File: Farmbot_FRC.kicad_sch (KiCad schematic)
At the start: 3 parts, among them J1 XT60-M, U1 NEO-6M-GPS

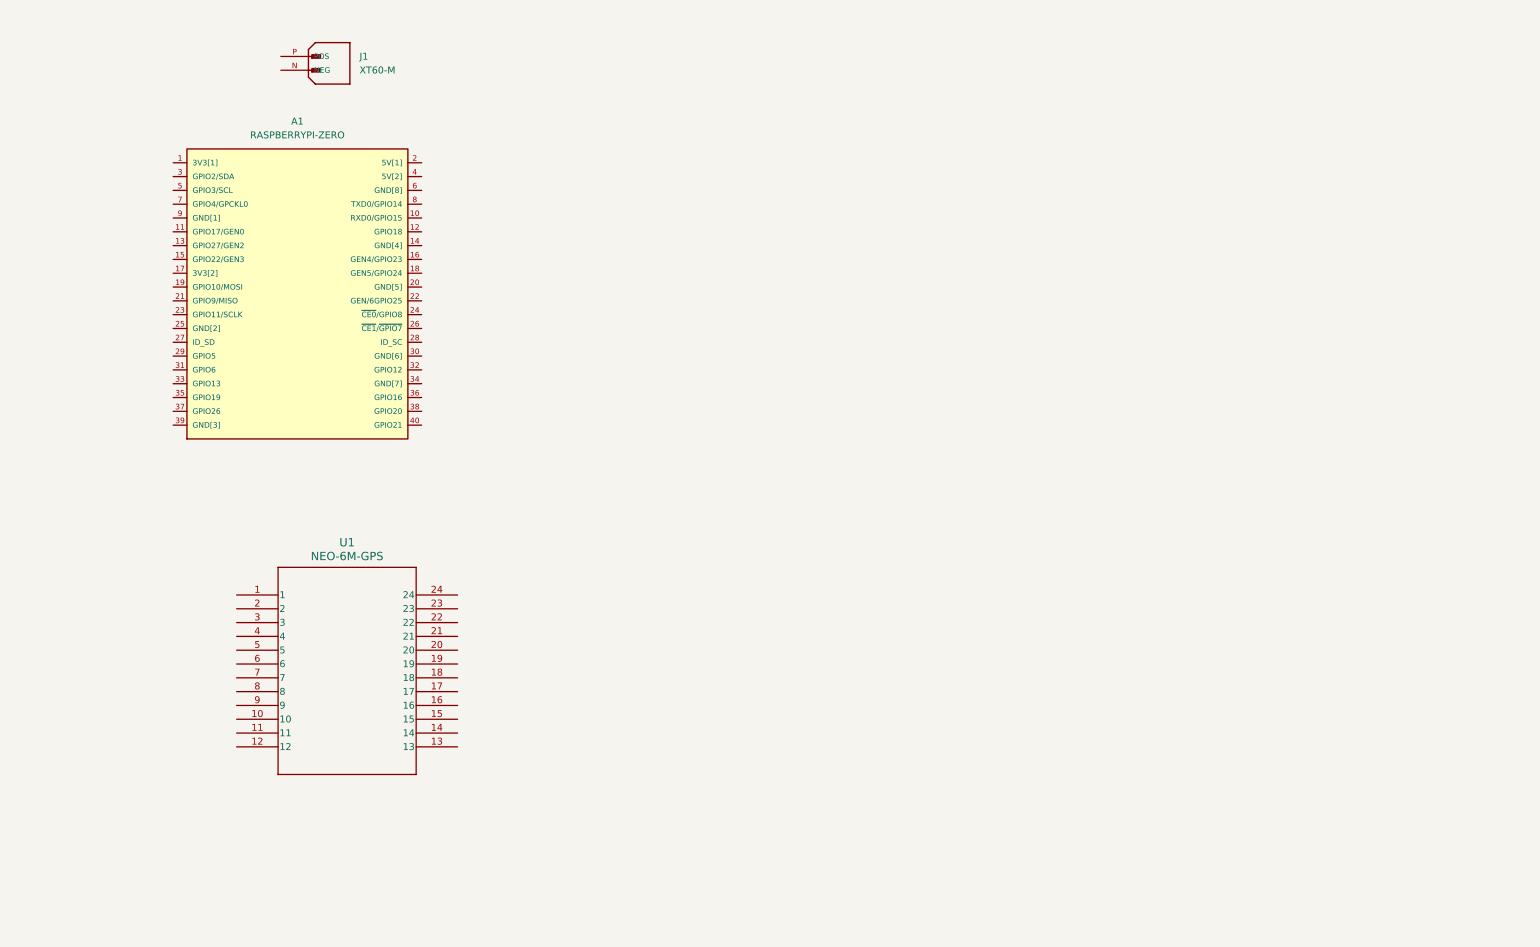
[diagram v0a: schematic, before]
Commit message: Added basic components
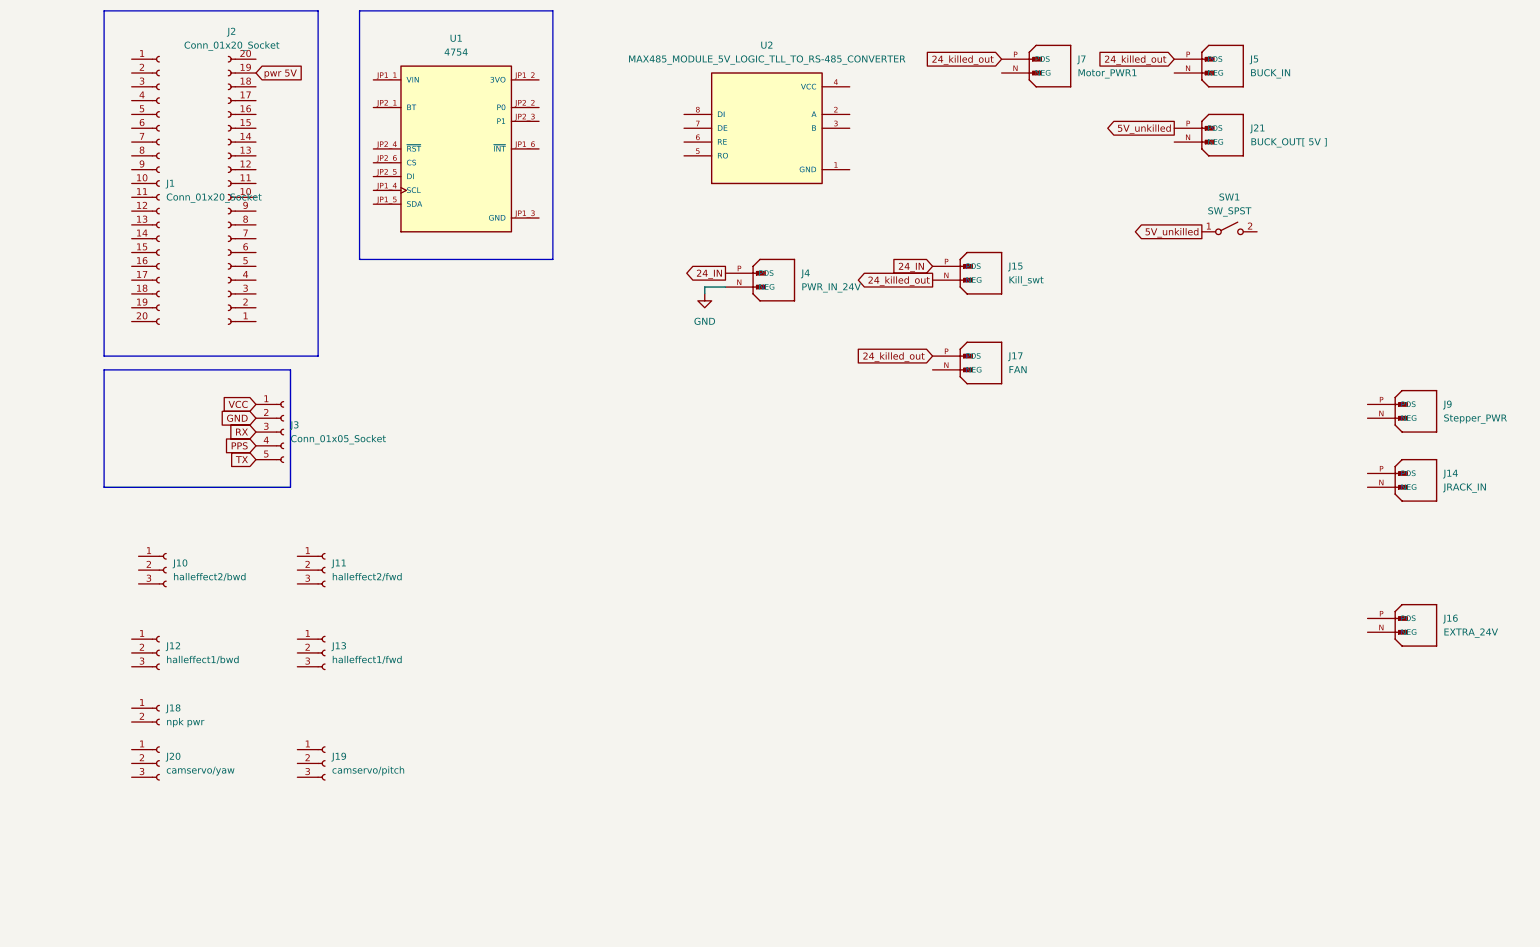
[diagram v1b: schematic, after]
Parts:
- removed A1: RASPBERRYPI-ZERO, RASPBERRYPI-ZERO:RASPBERRYPI-ZERO_RPI-ZERO, symbol RASPBERRYPI-ZERO:RASPBERRYPI-ZERO
- removed J1: XT60-M, XT60-M:AMASS_XT60-M, symbol XT60-M:XT60-M
- removed U1: NEO-6M-GPS, SON_6M-GPS_UBL, symbol gps neo 6m:NEO-6M-GPS
- added J1, J2: Conn_01x20_Socket, symbol Connector:Conn_01x20_Socket
- added J10: halleffect2/bwd, symbol Connector:Conn_01x03_Socket
- added J11: halleffect2/fwd, symbol Connector:Conn_01x03_Socket
- added J12: halleffect1/bwd, symbol Connector:Conn_01x03_Socket
- added J13: halleffect1/fwd, symbol Connector:Conn_01x03_Socket
- added J14: JRACK_IN, XT60-M:AMASS_XT60-M, symbol XT60-M:XT60-M
- added J15: Kill_swt, XT60-M:AMASS_XT60-M, symbol XT60-M:XT60-M
- added J16: EXTRA_24V, XT60-M:AMASS_XT60-M, symbol XT60-M:XT60-M
- added J17: FAN, XT60-M:AMASS_XT60-M, symbol XT60-M:XT60-M
- added J18: npk pwr, symbol Connector:Conn_01x02_Socket
- added J19: camservo/pitch, symbol Connector:Conn_01x03_Socket
- added J20: camservo/yaw, symbol Connector:Conn_01x03_Socket
- added J21: BUCK_OUT[ 5V ], XT60-M:AMASS_XT60-M, symbol XT60-M:XT60-M
- added J3: Conn_01x05_Socket, symbol Connector:Conn_01x05_Socket
- added J4: PWR_IN_24V, XT60-M:AMASS_XT60-M, symbol XT60-M:XT60-M
- added J5: BUCK_IN, XT60-M:AMASS_XT60-M, symbol XT60-M:XT60-M
- added J7: Motor_PWR1, XT60-M:AMASS_XT60-M, symbol XT60-M:XT60-M
- added J9: Stepper_PWR, XT60-M:AMASS_XT60-M, symbol XT60-M:XT60-M
- added SW1: SW_SPST, symbol Switch:SW_SPST
- added U1: 4754, 4754:MODULE_4754, symbol 4754:4754
- added U2: MAX485_MODULE_5V_LOGIC_TLL_TO_RS-485_CONVERTER, MAX485_MODULE_5V_LOGIC_TLL_TO_RS-485_CONVERTER:MODULE_MAX485_MODULE_5V_LOGIC_TLL_TO_RS-485_CONVERTER, symbol max rs485(npk):MAX485_MODULE_5V_LOGIC_TLL_TO_RS-485_CONVERTER
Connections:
- new net 24_IN: J15.P (POS), J4.P (POS)
- new net 24_killed_out: J15.N (NEG), J17.P (POS), J5.P (POS), J7.P (POS)
- new net 5V_unkilled: J21.P (POS), SW1.1 (A)
- new net GND: J3.2 (Pin_2), J4.N (NEG)
- new net PPS: J3.4 (Pin_4)
- new net RX: J3.3 (Pin_3)
- new net TX: J3.5 (Pin_5)
- new net VCC: J3.1 (Pin_1)
- new net pwr 5V: J2.19 (Pin_19)

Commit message: made changes to the pcb
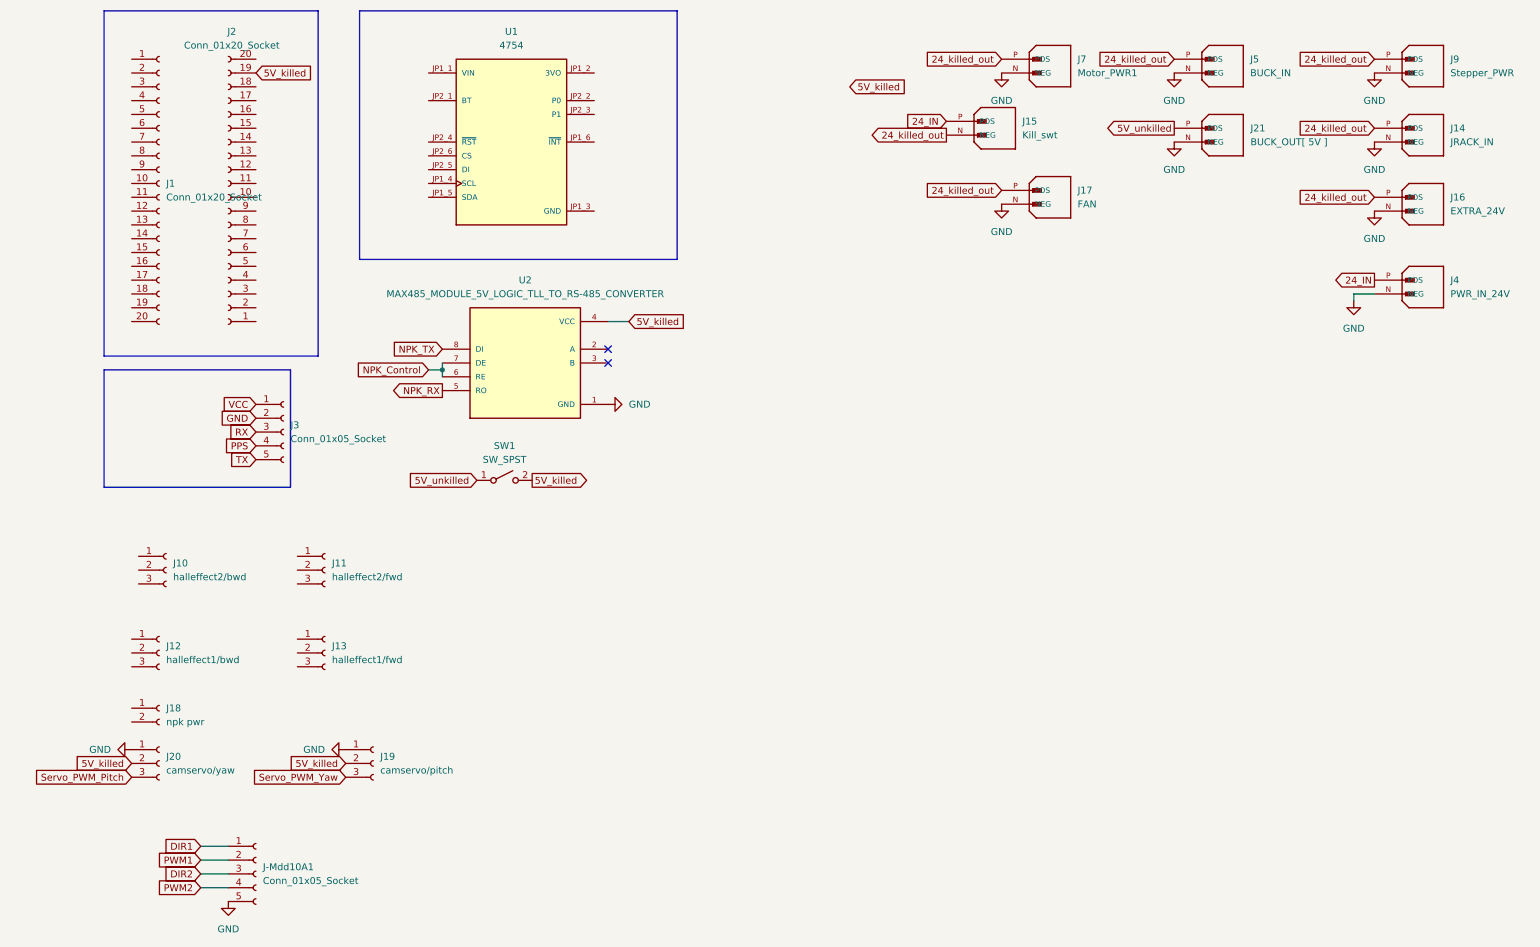
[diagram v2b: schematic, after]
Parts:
- added J-Mdd10A1: Conn_01x05_Socket, Connector_JST:JST_EH_B5B-EH-A_1x05_P2.50mm_Vertical, symbol Connector:Conn_01x05_Socket
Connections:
- net pwr 5V is gone; now on net 5V_killed: J2.19 (Pin_19)
- net 24_killed_out: now also J14.P (POS), J16.P (POS), J9.P (POS)
- net GND: now also J14.N (NEG), J16.N (NEG), J17.N (NEG), J19.1 (Pin_1), J20.1 (Pin_1), J21.N (NEG), J5.N (NEG), J7.N (NEG), J9.N (NEG), U2.1 (GND), J-Mdd10A1.5 (Pin_5)
- net 5V_killed: now reaches J20.2 (Pin_2)
- net 5V_killed: now also J19.2 (Pin_2), SW1.2 (B), U2.4 (VCC)
- net Servo_PWM_Pitch: now reaches J20.3 (Pin_3)
- net NPK_RX: now reaches U2.5 (RO)
- net NPK_Control: now reaches U2.6 (RE)
- net NPK_Control: now also U2.7 (DE)
- net NPK_TX: now reaches U2.8 (DI)
- net Servo_PWM_Yaw: now reaches J19.3 (Pin_3)
- new net DIR1: J-Mdd10A1.1 (Pin_1)
- new net DIR2: J-Mdd10A1.3 (Pin_3)
- new net PWM1: J-Mdd10A1.2 (Pin_2)
- new net PWM2: J-Mdd10A1.4 (Pin_4)
- no-connect marks 0 -> 2
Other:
- moved on the sheet: J14, J15, J16, J17, J19, J4, J9, SW1, U1, U2
